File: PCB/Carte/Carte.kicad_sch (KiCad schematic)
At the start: 5 parts, among them U1 LM2596S-5, U2 MPU-6050

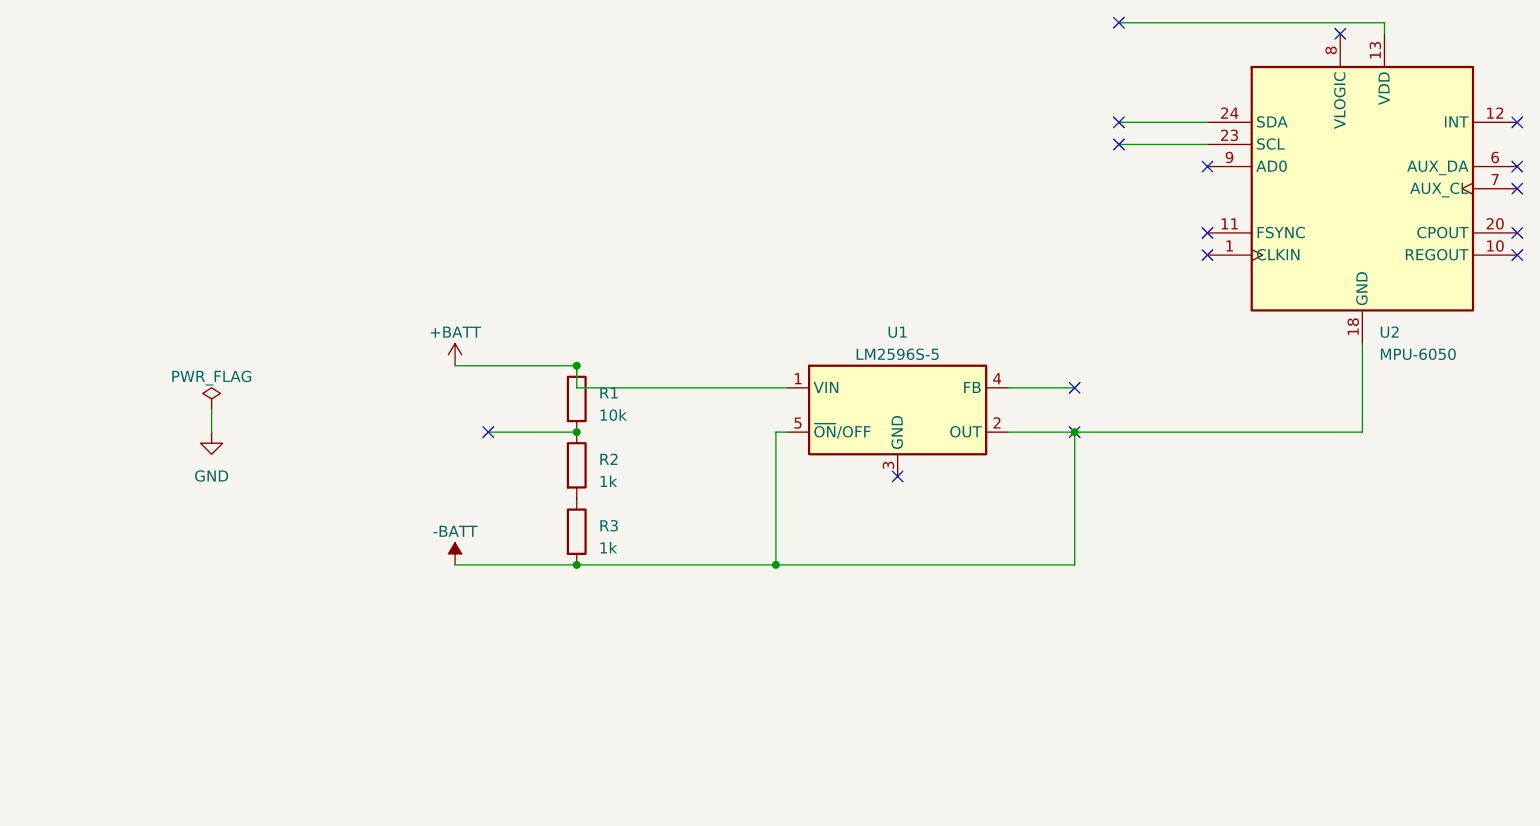
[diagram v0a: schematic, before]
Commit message: PCB
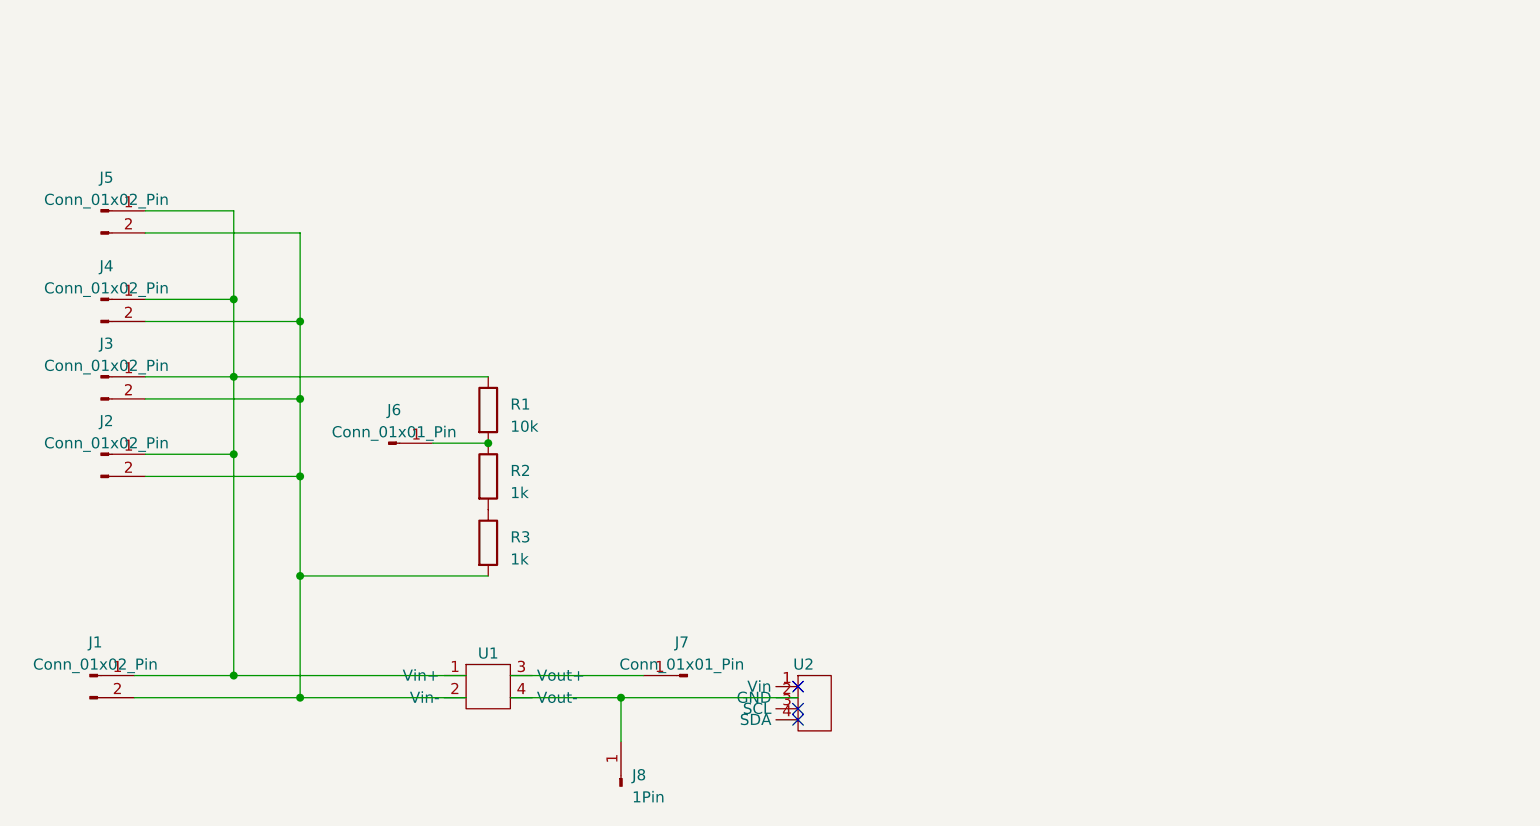
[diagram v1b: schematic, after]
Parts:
- removed U1: LM2596S-5, Package_TO_SOT_SMD:TO-263-5_TabPin3, symbol my_lib:LM2596S-5
- added J1, J2, J3, J4, J5: Conn_01x02_Pin, my_lib:2Pin, symbol my_lib:Conn_01x02_Pin
- added J6, J7: Conn_01x01_Pin, my_lib:1Pin, symbol my_lib:Conn_01x01_Pin
- added J8: 1Pin, my_lib:1Pin, symbol my_lib:1Pin
- added U1: ~, my_lib:LM2596S, symbol my_lib:LM2596
- R1, R2, R3: footprint (none) -> my_lib:R
- U2: value MPU-6050 -> ~; footprint Sensor_Motion:InvenSense_QFN-24_4x4mm_P0.5mm -> my_lib:MPU-6050
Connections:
- net at U2.2 (GND): now also J8.1 (Pin_1), U1.4 (Vout-)
- net at R1.2, R2.1: now also J6.1 (Pin_1)
- net +BATT: no longer names the net of R1.1
- net +BATT: now also J1.1 (Pin_1), J2.1 (Pin_1), J3.1 (Pin_1), J4.1 (Pin_1), J5.1 (Pin_1), U1.1 (Vin+)
- net -BATT: no longer names the net of R3.2
- net -BATT: now also J1.2 (Pin_2), J2.2 (Pin_2), J3.2 (Pin_2), J4.2 (Pin_2), J5.2 (Pin_2), U1.2 (Vin-); no longer U2.18 (GND)
- new net: J7.1 (Pin_1), U1.3 (Vout+)
- no-connect marks 16 -> 3
